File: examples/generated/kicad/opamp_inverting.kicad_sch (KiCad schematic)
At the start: 6 parts

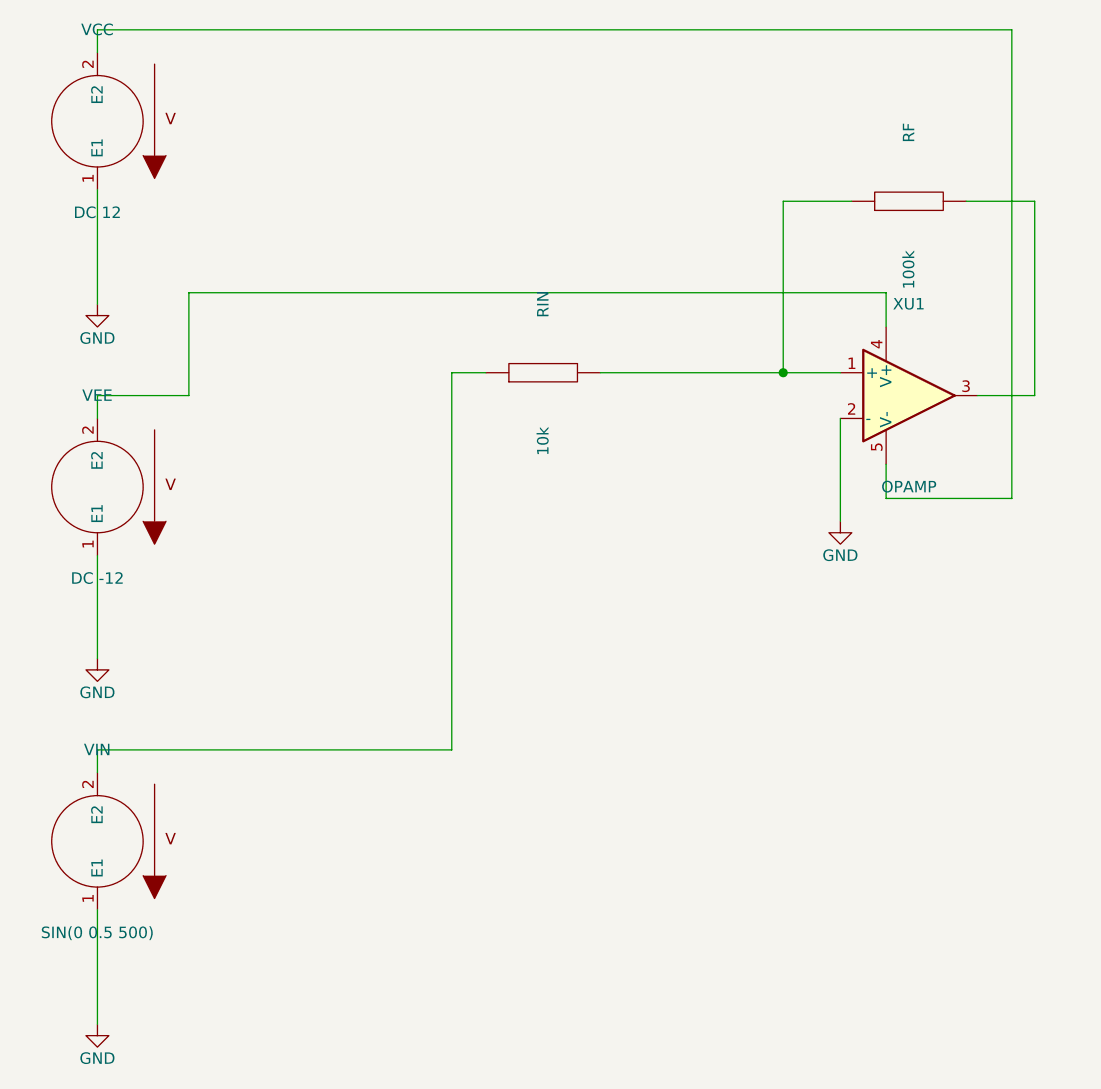
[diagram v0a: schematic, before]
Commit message: Refactor further.
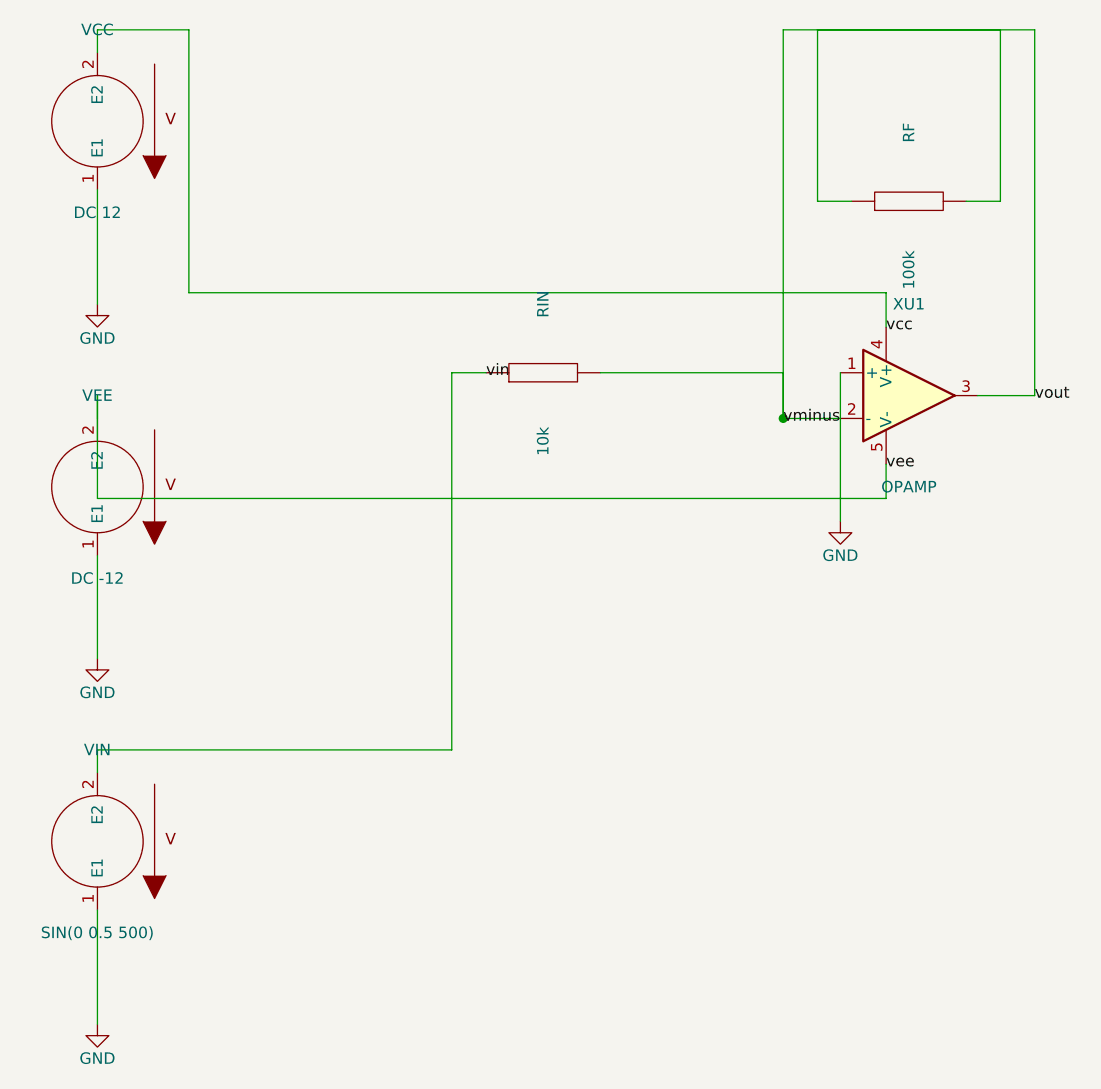
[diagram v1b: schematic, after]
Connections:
- net GND: now also XU1.1 (+); no longer XU1.2 (-)
- net vcc: now reaches VCC.2 (E2)
- net vcc: now also XU1.4 (V+); no longer XU1.5 (V-)
- net vminus: now reaches RF.1, RIN.2
- net vminus: now also RF.2, XU1.2 (-), XU1.3; no longer XU1.1 (+)
- net vee: now reaches VEE.2 (E2)
- net vee: now also XU1.5 (V-); no longer XU1.4 (V+)
- net vin: now reaches RIN.1, VIN.2 (E2)
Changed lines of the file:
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@@
     )
+  )
+  (label "vin" (at 123.19 87.63 0)
+    (effects (font (size 1.27 1.27)))
+  )
+  (label "vminus" (at 156.21 92.71 0)
+    (effects (font (size 1.27 1.27)))
+  )
+  (label "vout" (at 184.15 90.17 0)
+    (effects (font (size 1.27 1.27)))
+  )
+  (label "vcc" (at 167.64 82.55 0)
+    (effects (font (size 1.27 1.27)))
+  )
+  (label "vee" (at 167.64 97.79 0)
+    (effects (font (size 1.27 1.27)))
   )
   (wire (pts (xy 80.01 67.31) (xy 80.01 80.01))
@@
     (stroke (width 0) (type solid) (color 0 0 0 0))
   )
-  (wire (pts (xy 162.56 92.71) (xy 162.56 104.14))
+  (wire (pts (xy 162.56 87.63) (xy 162.56 104.14))
     (stroke (width 0) (type solid) (color 0 0 0 0))
   )
@@
     (stroke (width 0) (type solid) (color 0 0 0 0))
   )
-  (wire (pts (xy 162.56 87.63) (xy 156.21 87.63))
+  (wire (pts (xy 156.21 87.63) (xy 156.21 92.71))
     (stroke (width 0) (type solid) (color 0 0 0 0))
   )
-  (wire (pts (xy 163.83 68.58) (xy 156.21 68.58))
+  (wire (pts (xy 162.56 92.71) (xy 156.21 92.71))
     (stroke (width 0) (type solid) (color 0 0 0 0))
   )
-  (wire (pts (xy 156.21 68.58) (xy 156.21 87.63))
+  (wire (pts (xy 176.53 68.58) (xy 180.34 68.58))
+    (stroke (width 0) (type solid) (color 0 0 0 0))
+  )
+  (wire (pts (xy 180.34 68.58) (xy 180.34 49.53))
+    (stroke (width 0) (type solid) (color 0 0 0 0))
+  )
+  (wire (pts (xy 180.34 49.53) (xy 156.21 49.53))
+    (stroke (width 0) (type solid) (color 0 0 0 0))
+  )
+  (wire (pts (xy 156.21 49.53) (xy 156.21 92.71))
     (stroke (width 0) (type solid) (color 0 0 0 0))
   )
@@
     (stroke (width 0) (type solid) (color 0 0 0 0))
   )
-  (wire (pts (xy 176.53 68.58) (xy 184.15 68.58))
+  (wire (pts (xy 163.83 68.58) (xy 160.02 68.58))
     (stroke (width 0) (type solid) (color 0 0 0 0))
   )
-  (wire (pts (xy 184.15 68.58) (xy 184.15 90.17))
+  (wire (pts (xy 160.02 68.58) (xy 160.02 49.53))
     (stroke (width 0) (type solid) (color 0 0 0 0))
   )
-  (wire (pts (xy 167.64 97.79) (xy 167.64 101.60))
+  (wire (pts (xy 160.02 49.53) (xy 184.15 49.53))
     (stroke (width 0) (type solid) (color 0 0 0 0))
   )
-  (wire (pts (xy 167.64 101.60) (xy 181.61 101.60))
-    (stroke (width 0) (type solid) (color 0 0 0 0))
-  )
-  (wire (pts (xy 181.61 101.60) (xy 181.61 49.53))
-    (stroke (width 0) (type solid) (color 0 0 0 0))
-  )
-  (wire (pts (xy 181.61 49.53) (xy 80.01 49.53))
-    (stroke (width 0) (type solid) (color 0 0 0 0))
-  )
-  (wire (pts (xy 80.01 49.53) (xy 80.01 52.07))
+  (wire (pts (xy 184.15 49.53) (xy 184.15 90.17))
     (stroke (width 0) (type solid) (color 0 0 0 0))
   )
@@
     (stroke (width 0) (type solid) (color 0 0 0 0))
   )
-  (wire (pts (xy 90.17 78.74) (xy 90.17 90.17))
+  (wire (pts (xy 90.17 78.74) (xy 90.17 49.53))
     (stroke (width 0) (type solid) (color 0 0 0 0))
   )
-  (wire (pts (xy 90.17 90.17) (xy 80.01 90.17))
+  (wire (pts (xy 90.17 49.53) (xy 80.01 49.53))
+    (stroke (width 0) (type solid) (color 0 0 0 0))
+  )
+  (wire (pts (xy 80.01 49.53) (xy 80.01 52.07))
+    (stroke (width 0) (type solid) (color 0 0 0 0))
+  )
+  (wire (pts (xy 167.64 97.79) (xy 167.64 101.60))
+    (stroke (width 0) (type solid) (color 0 0 0 0))
+  )
+  (wire (pts (xy 167.64 101.60) (xy 80.01 101.60))
+    (stroke (width 0) (type solid) (color 0 0 0 0))
+  )
+  (wire (pts (xy 80.01 101.60) (xy 80.01 90.17))
     (stroke (width 0) (type solid) (color 0 0 0 0))
   )
@@
     (stroke (width 0) (type solid) (color 0 0 0 0))
   )
-  (junction (at 156.21 87.63) (diameter 1.016) (color 0 0 0 0))
+  (junction (at 156.21 92.71) (diameter 1.016) (color 0 0 0 0))
   (sheet_instances
     (path "/" (page "1"))
